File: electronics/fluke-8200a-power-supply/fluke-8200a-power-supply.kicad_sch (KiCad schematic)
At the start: 66 parts, among them J1 Conn_01x08, J2 Conn_01x03, Q1 NPN, Q10 NPN, Q11 2N3055, Q12 NPN, Q13 NPN, Q2 NPN, Q3 NPN, Q4 NPN, Q5 NPN, Q6 NPN, Q7 NPN

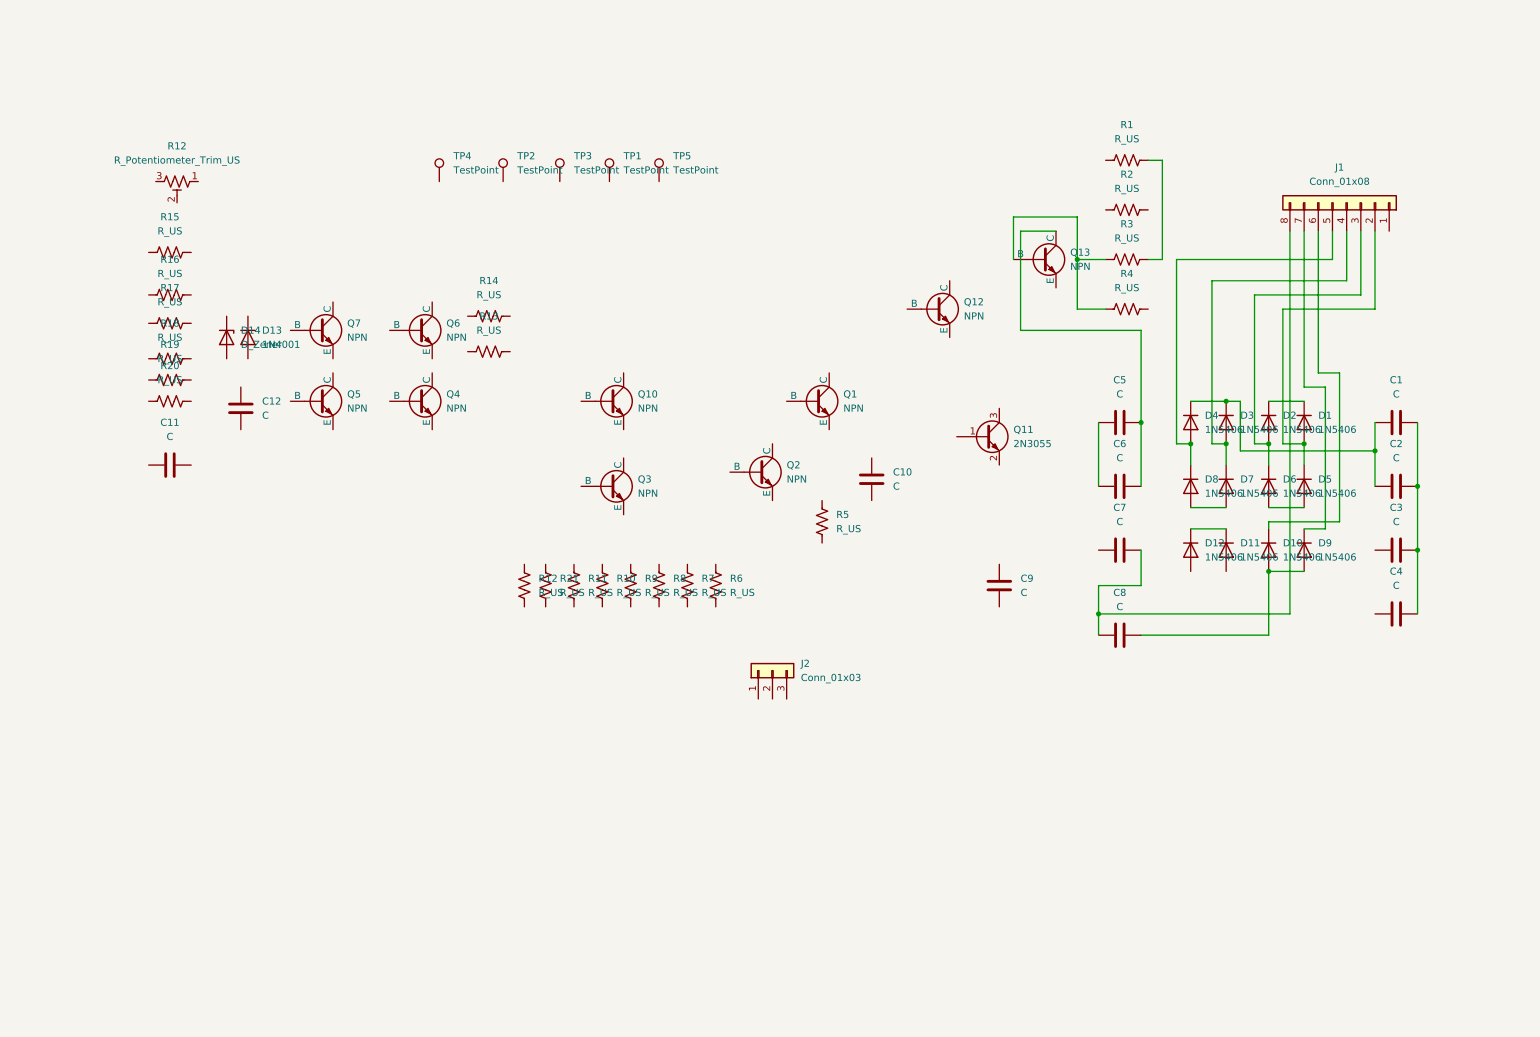
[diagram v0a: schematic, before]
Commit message: only need correct transistors now
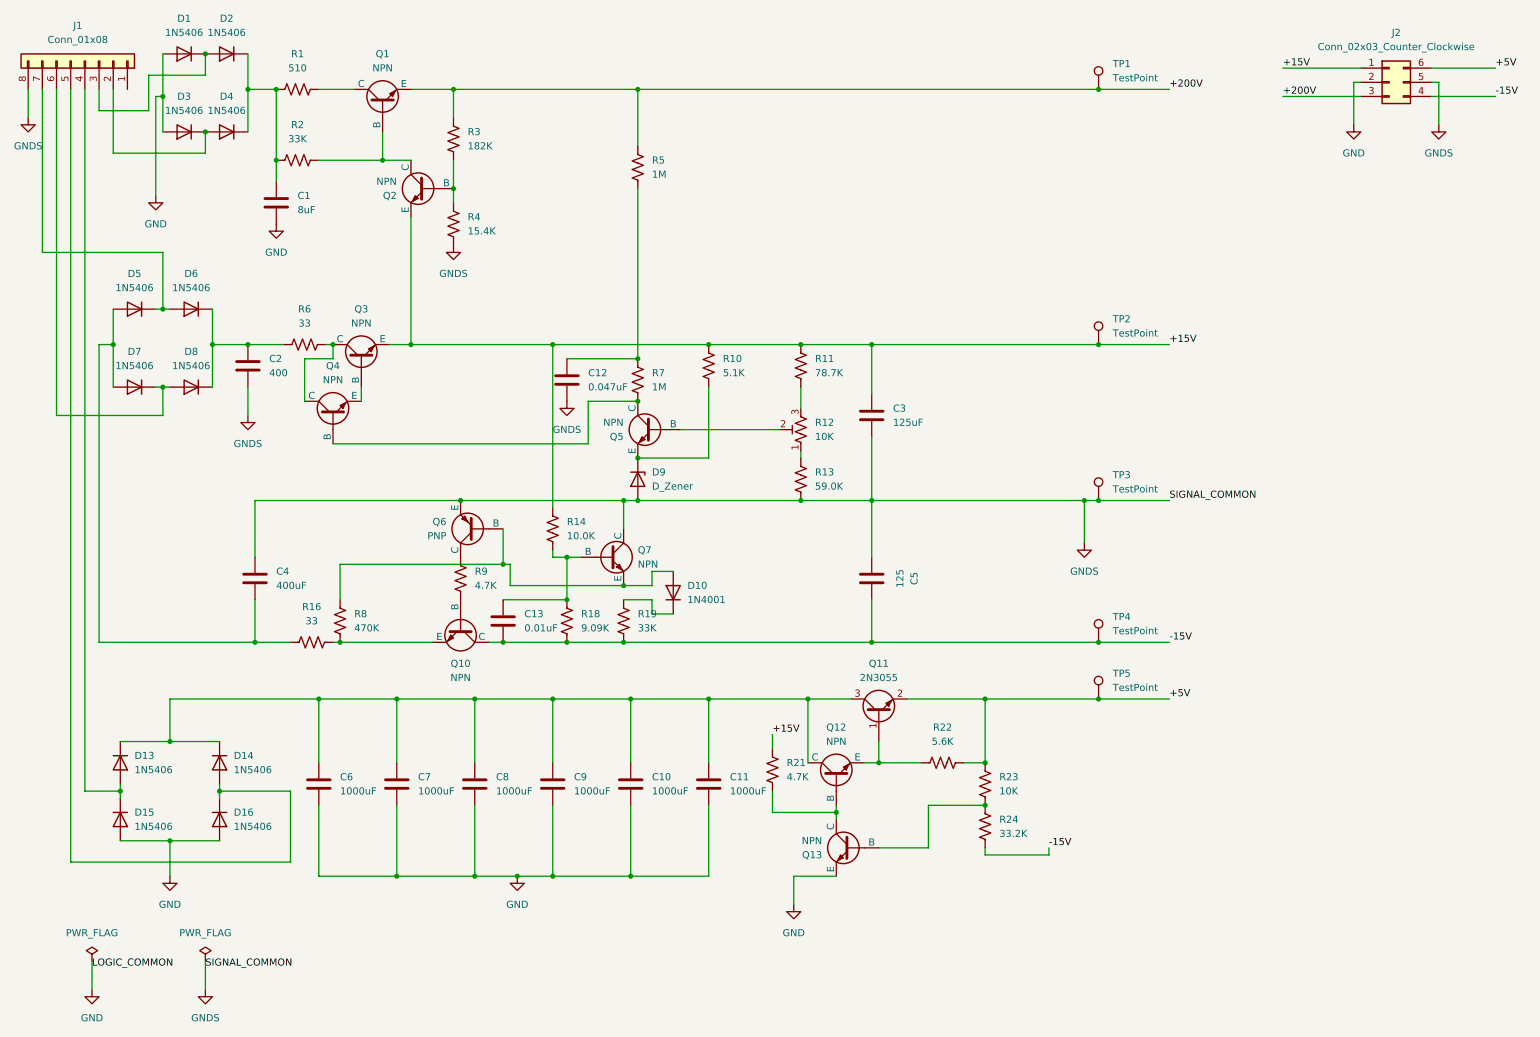
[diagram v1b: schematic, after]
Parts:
- removed J2: Conn_01x03, symbol Connector_Generic:Conn_01x03
- removed Q6: NPN, symbol Simulation_SPICE:NPN
- removed R15: R_US, symbol Device:R_US
- added C13: 0.01uF, symbol Device:C
- added J2: Conn_02x03_Counter_Clockwise, symbol Connector_Generic:Conn_02x03_Counter_Clockwise
- added Q6: PNP, symbol Simulation_SPICE:PNP
- C1: value C -> 8uF
- C10, C11, C6, C7, C8, C9: value C -> 1000uF
- C12: value C -> 0.047uF
- C2: value C -> 400
- C3: value C -> 125uF
- C4: value C -> 400uF
- C5: value C -> 125
- R1: value R_US -> 510
- R10: value R_US -> 5.1K
- R11: value R_US -> 78.7K
- R12: value R_Potentiometer_Trim_US -> 10K
- R13: renamed from R21; value R_US -> 59.0K
- R14: value R_US -> 10.0K
- R16, R6: value R_US -> 33
- R18: renamed from R12; value R_US -> 9.09K
- R19: renamed from R13; value R_US -> 33K
- R2: value R_US -> 33K
- R21: renamed from R20; value R_US -> 4.7K
- R22: renamed from R19; value R_US -> 5.6K
- R23: renamed from R18; value R_US -> 10K
- R24: renamed from R17; value R_US -> 33.2K
- R3: value R_US -> 182K
- R4: value R_US -> 15.4K
- R5, R7: value R_US -> 1M
- R8: value R_US -> 470K
- R9: value R_US -> 4.7K
- renumbered D13 to D10, D9 to D13, D10 to D14, D12 to D15, D11 to D16, D14 to D9
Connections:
- net at D15.1 (K): now also D13.2 (A), J1.4 (Pin_4); no longer D16.1 (K)
- net GND: now reaches D15.2 (A)
- net GND: now also C1.1, C10.2, C11.2, C6.2, C7.2, C8.2, C9.2, D1.2 (A), D16.2 (A), D3.2 (A), Q13.3 (E), J2.2 (Pin_2)
- net +5V: now reaches TP5.1
- net +5V: now also Q11.2 (E), R22.2, R23.2, J2.6 (Pin_6)
- net GNDS: now reaches TP3.1
- net GNDS: now also C12.1, C2.1, C3.1, C4.2, C5.1, D9.2 (A), J1.8 (Pin_8), Q7.1 (C), R13.2, R4.1, J2.5 (Pin_5), Q6.3 (E)
- net at C7.1: now also C10.1, C11.1, C6.1, C8.1, C9.1, D13.1 (K), D14.1 (K), Q11.3 (C), Q12.1 (C)
- net +200V: now reaches R5.1
- net +200V: now also Q1.3 (E), R3.2, TP1.1, J2.3 (Pin_3)
- net at R5.2: now also C12.2, R7.1
- net at R23.1: now also Q13.2 (B), R24.2
- net at Q5.1 (C): now also Q4.2 (B), R7.2
- net at Q5.2 (B): now also R12.2
- net at Q5.3 (E): now also D9.1 (K), R10.2
- net at R8.1: now also D10.2 (A), Q7.3 (E), Q6.2 (B)
- net at R8.2: now also Q10.3 (E), R16.2
- net at R1.1: now also C1.2, D2.1 (K), D4.1 (K), R2.1
- net at R1.2: now also Q1.1 (C); no longer R3.2
- net at R12.1: now also R13.1
- net at R12.3: now also R11.2
- net at D6.2 (A): now also D5.1 (K), J1.7 (Pin_7); no longer D5.2 (A)
- net at R22.1: now also Q11.1 (B), Q12.3 (E)
- net at D1.1 (K): now also D2.2 (A), J1.3 (Pin_3); no longer D2.1 (K)
- net at D7.2 (A): now also C4.1, D5.2 (A), R16.1; no longer D8.2 (A)
- net at Q1.2 (B): now also Q2.1 (C), R2.2
- net at R6.1: now also C2.2, D6.1 (K), D8.1 (K)
- net at R6.2: now also Q3.1 (C), Q4.1 (C)
- net at Q3.2 (B): now also Q4.3 (E)
- net +15V: now reaches Q3.3 (E)
- net +15V: now also C3.2, Q2.3 (E), R10.1, R11.1, R14.1, R21.2, TP2.1, J2.1 (Pin_1)
- net at D10.1 (K): now also R19.2
- net at R14.2: now also Q7.2 (B), R18.2, C13.1
- net at Q12.2 (B): now also Q13.1 (C), R21.1
- net -15V: now reaches R18.1
- net -15V: now also C5.2, Q10.1 (C), R19.1, R24.1, TP4.1, C13.2, J2.4 (Pin_4)
- net at J1.6 (Pin_6): now also D7.1 (K), D8.2 (A); no longer D14.1 (K)
- net at Q10.2 (B): now also R9.2
- net at R9.1: now also Q6.1 (C)
- net at Q2.2 (B): now also R3.1, R4.2
- new net: D3.1 (K), D4.2 (A), J1.2 (Pin_2)
- new net: D14.2 (A), D16.1 (K), J1.5 (Pin_5)
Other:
- moved on the sheet: C1, C12, C2, C3, C4, C5, C6, D1, D10, D13, D14, D15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
